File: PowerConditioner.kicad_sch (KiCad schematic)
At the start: 9 parts, among them J9 YK9010323000G, K1 BATT-EDLC, K2 SERIAL-PARALLEL, K3 OUTPUT, U3 IPB017N10N5LFATMA1, U5 IPB017N10N5LFATMA1

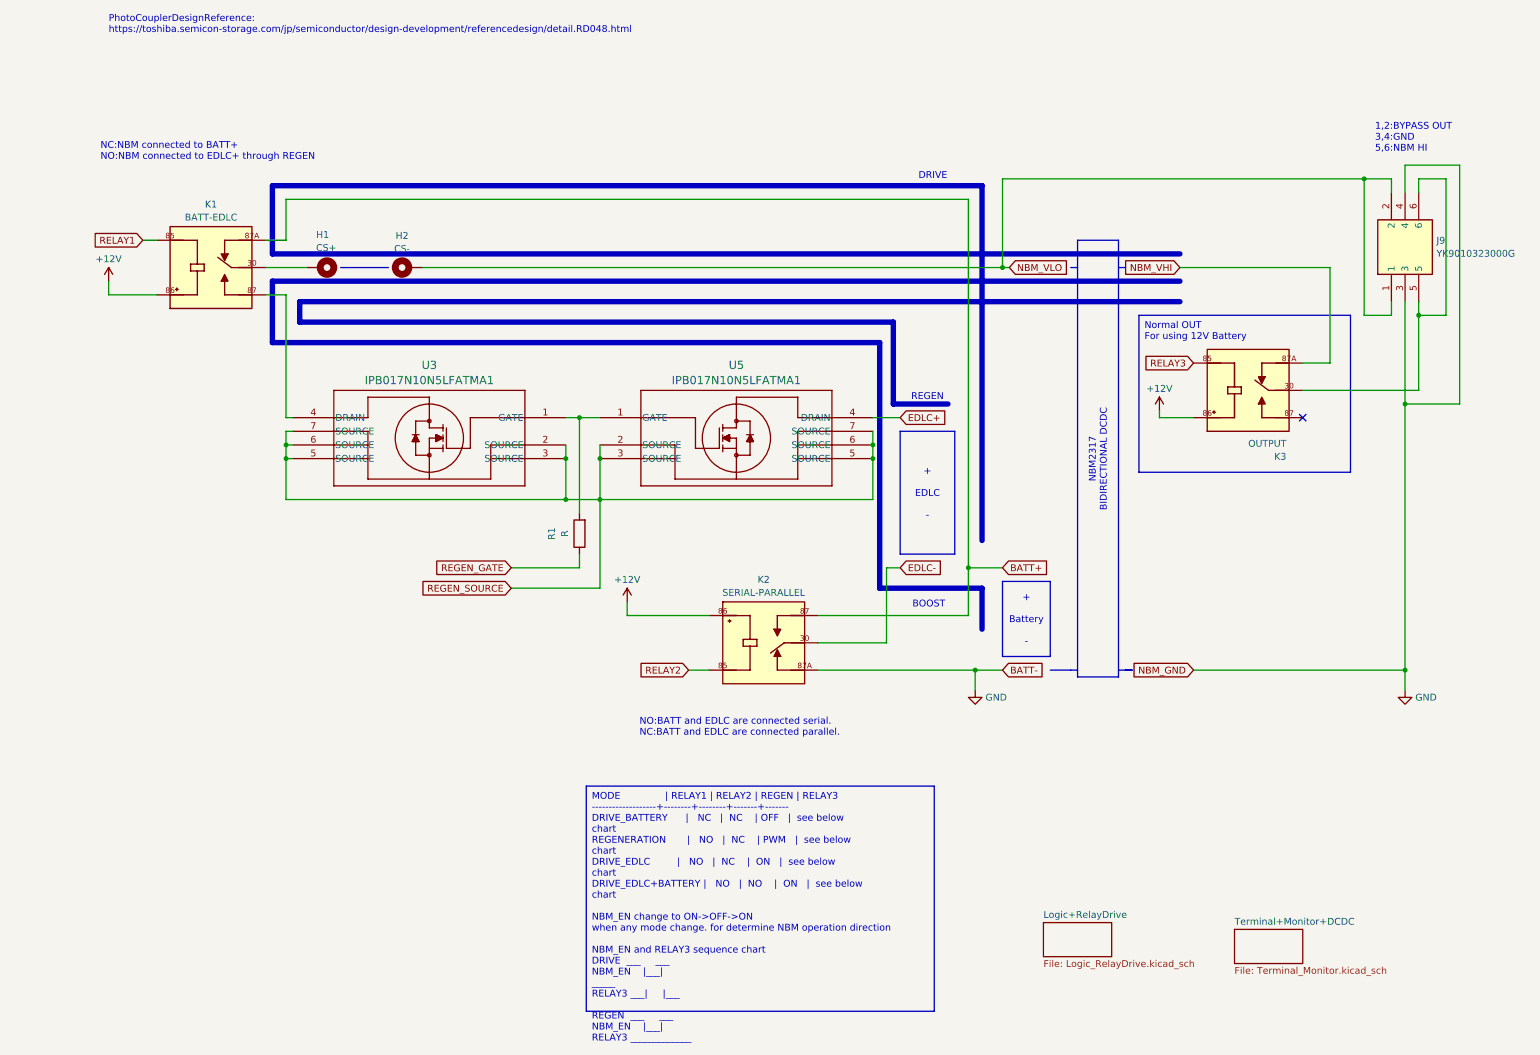
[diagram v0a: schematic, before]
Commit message: Order to JLCPCB
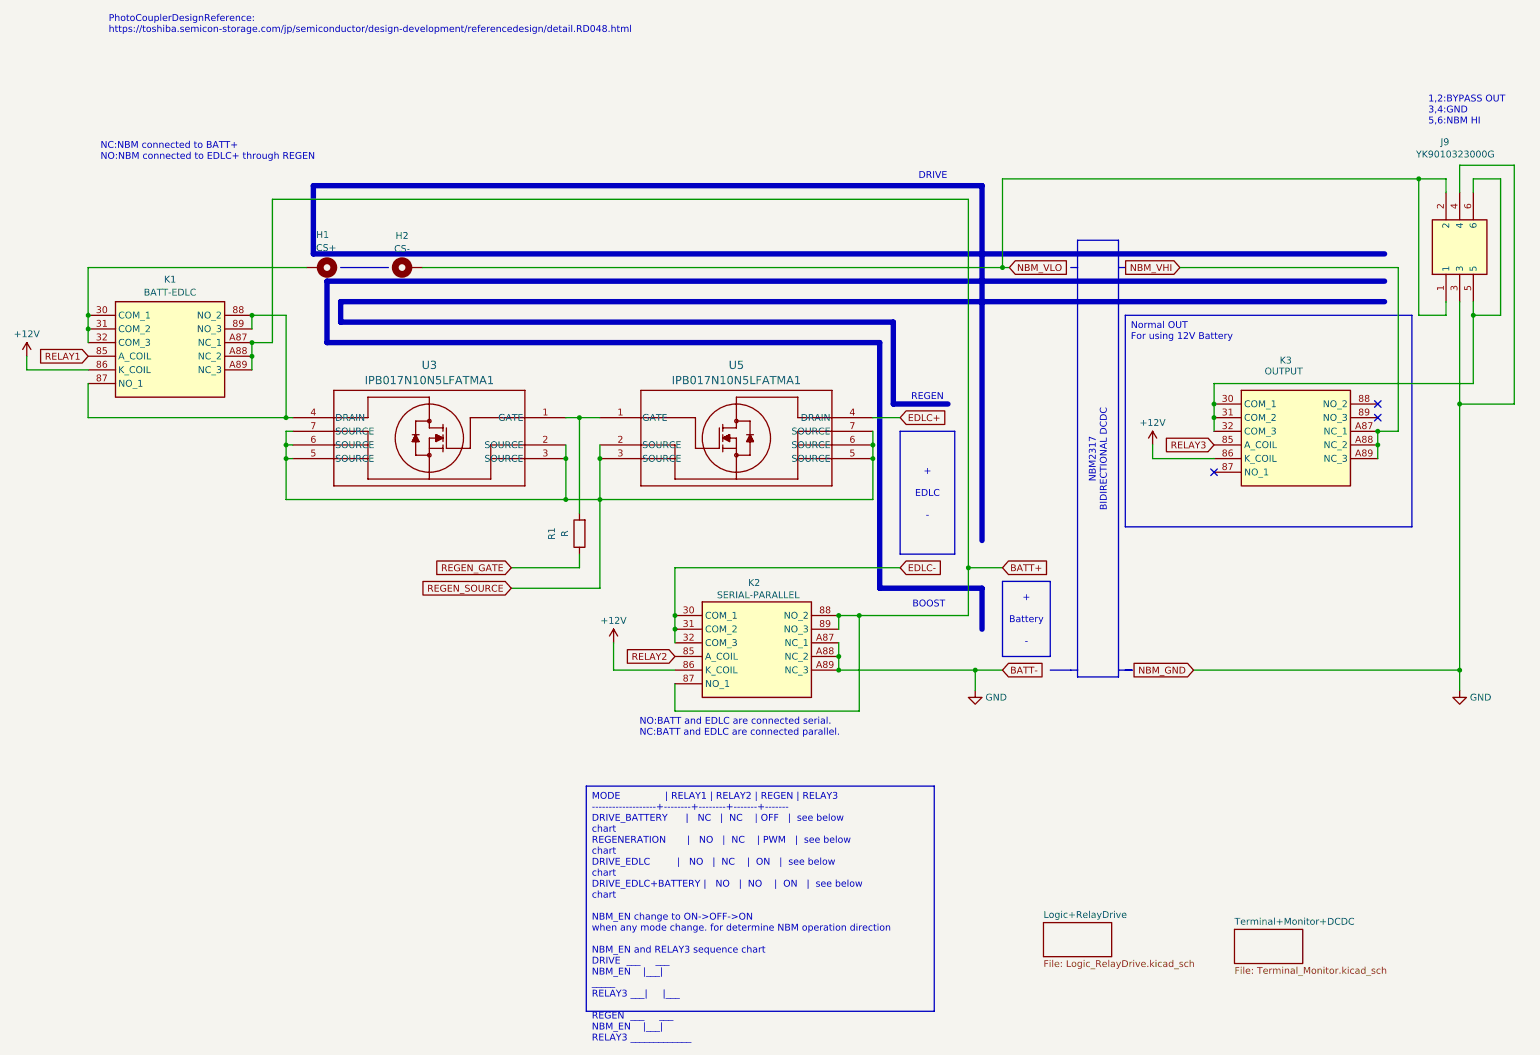
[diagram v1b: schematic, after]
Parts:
- K1, K2, K3: footprint 2-1904025-3:RELAY_2-1904025-3 -> A3K1CSP12VDC1.6D:A3K1CSP12VDC16D; symbol PC7150:2-1904025-3 -> A3K1CSP12VDC1.6D:A3K1CSP12VDC1.6D; Height (none) -> 24.5; Manufacturer_Name (none) -> CIT Relay & Switch; Manufacturer_Part_Number (none) -> A3K1CSP12VDC1.6D
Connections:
- net BATT+: now also K1.A87 (NC_1), K1.A88 (NC_2), K1.A89 (NC_3), K2.88 (NO_2), K2.89 (NO_3); no longer K1.87A
- net EDLC-: now also K2.31 (COM_2), K2.32 (COM_3)
- net GND: now also K2.A87 (NC_1), K2.A88 (NC_2), K2.A89 (NC_3); no longer K2.87A
- net NBM_VHI: now also K3.A87 (NC_1), K3.A88 (NC_2), K3.A89 (NC_3); no longer K3.87A
- net at H1.1, K1.30 (COM_1): now also K1.31 (COM_2), K1.32 (COM_3)
- net at J9.5, J9.6, K3.30 (COM_1): now also K3.31 (COM_2), K3.32 (COM_3)
- net at K1.87 (NO_1), U3.4 (DRAIN): now also K1.88 (NO_2), K1.89 (NO_3)
- no-connect marks 1 -> 3
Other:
- moved on the sheet: J9
